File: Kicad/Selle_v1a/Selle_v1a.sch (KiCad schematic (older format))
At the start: 0 parts

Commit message: Update Schematic
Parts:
- added C1: 10u, symbol Device:CP1
- added C2: 100u, symbol Device:CP1
- added C3, C4: 100n, symbol Device:C
- added D1: D_Schottky_AKA, symbol Device:D_Schottky_AKA
- added IC1: R-785.0-0.5, RECOM_R-785.0-0.5, symbol R-785.0-0.5:R-785.0-0.5
- added IC2: MCP2562, Package_SO:SOIC-8_3.9x4.9mm_P1.27mm, symbol Interface_CAN_LIN:MCP2562-E-SN
- added K1: ALIM, symbol Connector_Generic:Conn_01x02
- added K2: BUS CAN, symbol Connector_Generic:Conn_01x02
- added R1: 120, symbol Device:R
- added UC1: BluePill STM32, symbol YAAJ_STM32:BluePill_1
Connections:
- new net: IC2.6 (CANL), K2.2 (Pin_2), R1.2
- new net: IC2.7 (CANH), K2.1 (Pin_1), R1.1
- new net: C1.1, D1.2 (K), IC1.1 (+VIN)
- new net: D1.1 (A), D1.3 (A), K1.1 (Pin_1)
- new net +5V: C2.1, C4.2, IC1.3 (+VOUT), IC2.3 (VDD), UC1.18 (5V)
- new net CANRX: IC2.4 (RXD), UC1.8 (PA11)
- new net CANTX: IC2.1 (TXD), UC1.9 (PA12)
- new net GND: C1.2, C2.2, C3.2, C4.1, IC1.2 (GND), IC2.2 (VSS), IC2.8 (STBY), K1.2 (Pin_2), UC1.19 (GND), UC1.39 (GND), UC1.40 (GND)
- new net SCL: UC1.14 (PB6)
- new net SDA: UC1.15 (PB7)
- new net VCC: C3.1, IC2.5 (Vio), UC1.20 (3V3)

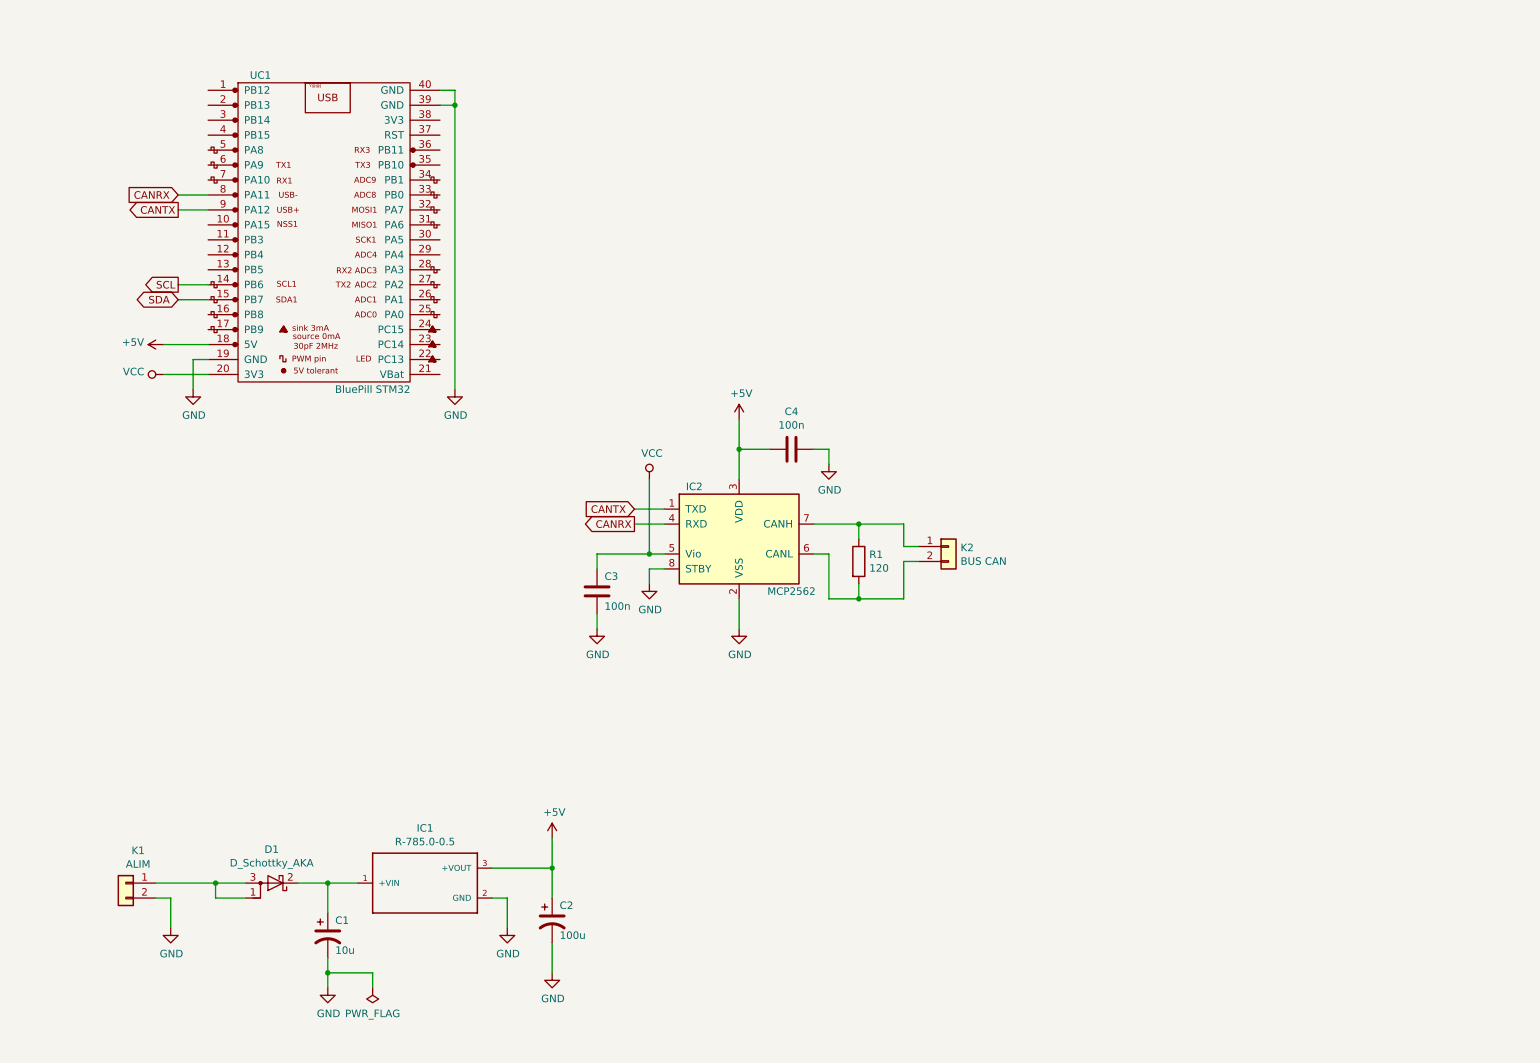
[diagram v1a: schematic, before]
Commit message: Update projet
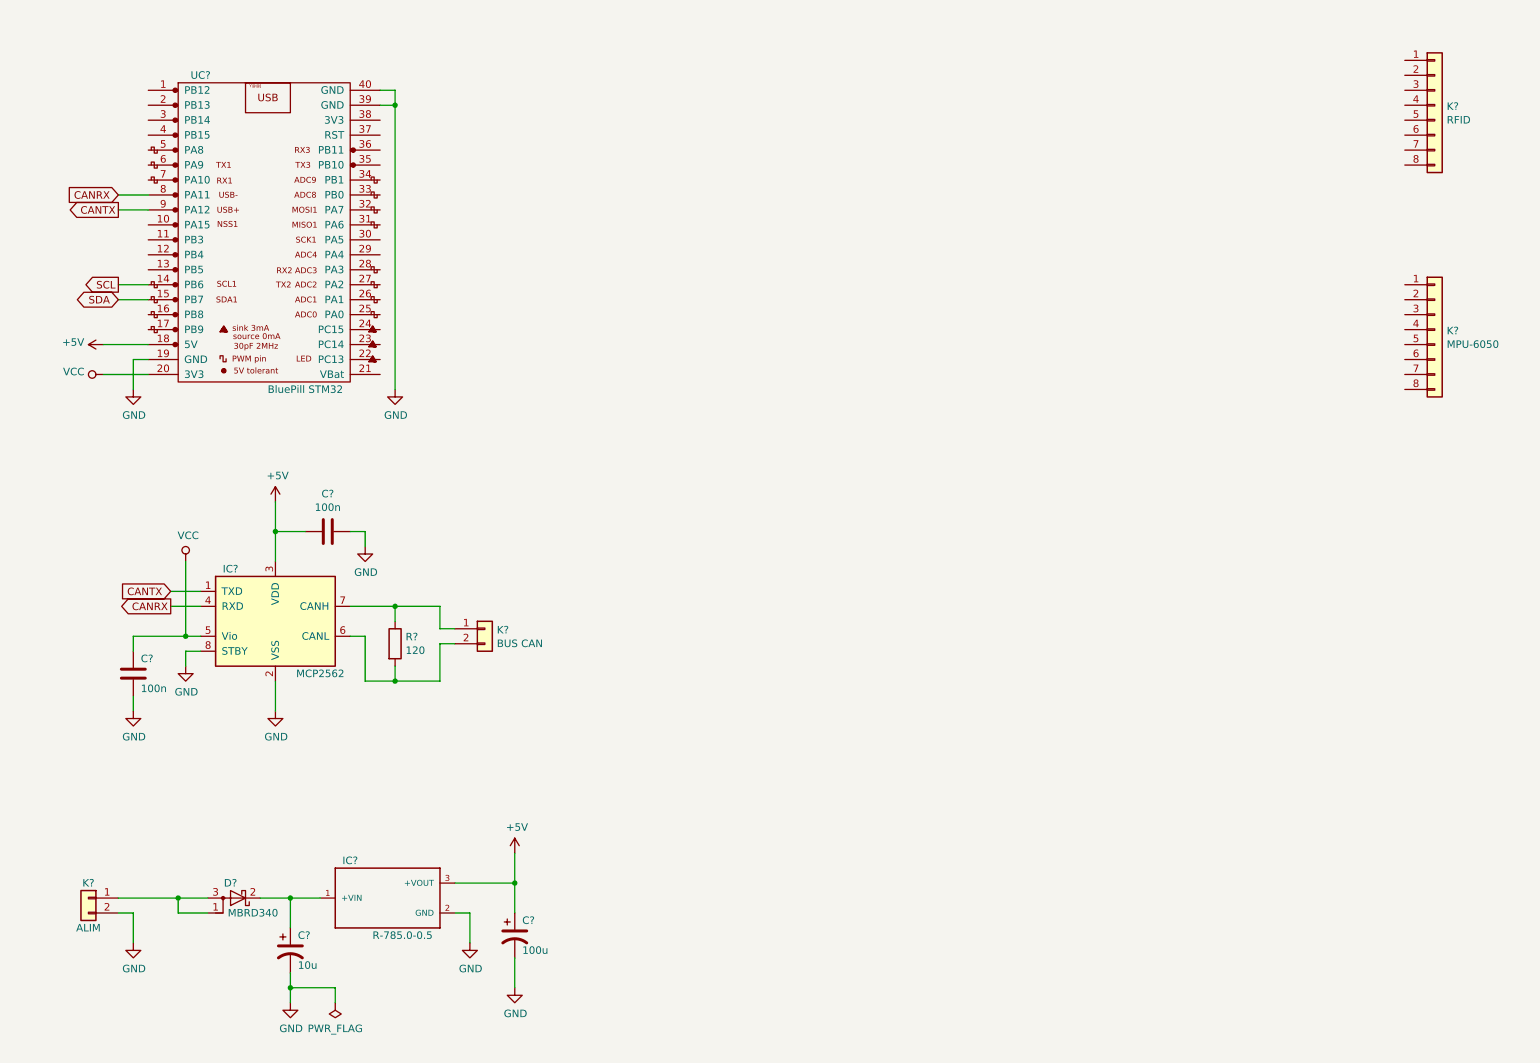
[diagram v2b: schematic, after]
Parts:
- added K?: RFID, symbol Connector_Generic:Conn_01x08
- added K?: MPU-6050, symbol Connector_Generic:Conn_01x08
- D?: renamed from D1; value D_Schottky_AKA -> MBRD340
- renumbered C4 to C?, C3 to C?, C1 to C?, C2 to C?, IC2 to IC?, IC1 to IC?, K1 to K?, K2 to K?, R1 to R?, UC1 to UC?
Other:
- moved on the sheet: C?, D?, IC?, K?, R?, UC?

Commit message: Update Schema
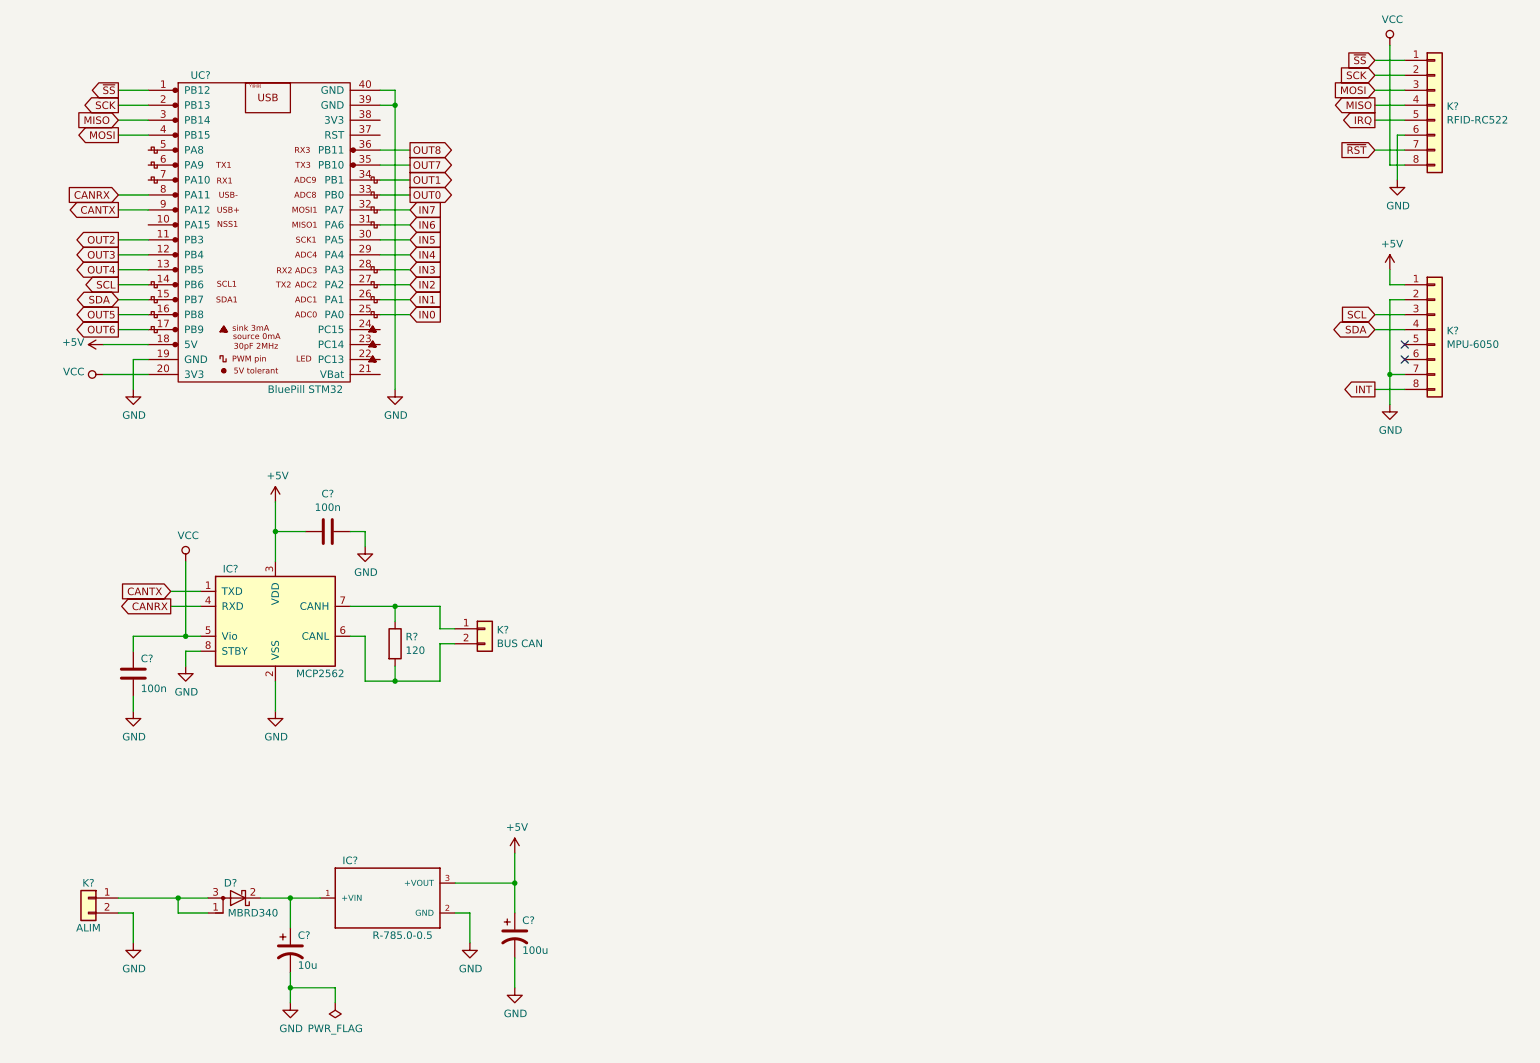
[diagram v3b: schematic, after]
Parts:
- K?: value RFID -> RFID-RC522
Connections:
- net +5V: now also K?.1 (Pin_1)
- net GND: now also K?.2 (Pin_2), K?.6 (Pin_6), K?.7 (Pin_7)
- net SCL: now also K?.3 (Pin_3)
- net SDA: now also K?.4 (Pin_4)
- net VCC: now also K?.8 (Pin_8)
- net ~SS: now reaches K?.1 (Pin_1)
- net ~SS: now also UC?.1 (PB12)
- net SCK: now reaches K?.2 (Pin_2)
- net SCK: now also UC?.2 (PB13)
- net MOSI: now reaches K?.3 (Pin_3)
- net MOSI: now also UC?.4 (PB15)
- net MISO: now reaches K?.4 (Pin_4)
- net MISO: now also UC?.3 (PB14)
- net IRQ: now reaches K?.5 (Pin_5)
- net ~RST: now reaches K?.7 (Pin_7)
- net INT: now reaches K?.8 (Pin_8)
- net OUT2: now reaches UC?.11 (PB3)
- net OUT3: now reaches UC?.12 (PB4)
- net OUT4: now reaches UC?.13 (PB5)
- net OUT5: now reaches UC?.16 (PB8)
- net OUT6: now reaches UC?.17 (PB9)
- net IN0: now reaches UC?.25 (PA0)
- net IN1: now reaches UC?.26 (PA1)
- net IN2: now reaches UC?.27 (PA2)
- net IN3: now reaches UC?.28 (PA3)
- net IN4: now reaches UC?.29 (PA4)
- net IN5: now reaches UC?.30 (PA5)
- net IN6: now reaches UC?.31 (PA6)
- net IN7: now reaches UC?.32 (PA7)
- net OUT0: now reaches UC?.33 (PB0)
- net OUT1: now reaches UC?.34 (PB1)
- net OUT7: now reaches UC?.35 (PB10)
- net OUT8: now reaches UC?.36 (PB11)
- no-connect marks 0 -> 2
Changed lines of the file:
@@
 P 10200 1300
 F 0 "K?" H 10280 1292 50  0000 L CNN
-F 1 "RFID" H 10280 1201 50  0000 L CNN
+F 1 "RFID-RC522" H 10280 1201 50  0000 L CNN
 F 2 "" H 10200 1300 50  0001 C CNN
 F 3 "~" H 10200 1300 50  0001 C CNN
@@
 	-1   0    0    1
 $EndComp
+Wire Wire Line
+	10000 1000 9800 1000
+Wire Wire Line
+	10000 1100 9800 1100
+Wire Wire Line
+	10000 1200 9800 1200
+Wire Wire Line
+	10000 1300 9800 1300
+$Comp
+L power:VCC #PWR?
+U 1 1 5E8C5F52
+P 9900 900
+F 0 "#PWR?" H 9900 750 50  0001 C CNN
+F 1 "VCC" H 9917 1073 50  0000 C CNN
+F 2 "" H 9900 900 50  0001 C CNN
+F 3 "" H 9900 900 50  0001 C CNN
+	1    9900 900
+	1    0    0    -1
+$EndComp
+$Comp
+L power:GND #PWR?
+U 1 1 5E8C663C
+P 9950 1800
+F 0 "#PWR?" H 9950 1550 50  0001 C CNN
+F 1 "GND" H 9955 1627 50  0000 C CNN
+F 2 "" H 9950 1800 50  0001 C CNN
+F 3 "" H 9950 1800 50  0001 C CNN
+	1    9950 1800
+	1    0    0    -1
+$EndComp
+Wire Wire Line
+	10000 1700 9900 1700
+Wire Wire Line
+	9900 1700 9900 900
+Wire Wire Line
+	10000 1500 9950 1500
+Wire Wire Line
+	9950 1500 9950 1800
+Wire Wire Line
+	10000 1600 9800 1600
+Text GLabel 9800 1000 0    50   Input ~ 0
+~SS
+Wire Wire Line
+	10000 1400 9800 1400
+Text GLabel 9800 1400 0    50   Output ~ 0
+IRQ
+Text GLabel 9800 1100 0    50   Input ~ 0
+SCK
+Text GLabel 9800 1200 0    50   Input ~ 0
+MOSI
+Text GLabel 9800 1300 0    50   Output ~ 0
+MISO
+Text GLabel 9800 1600 0    50   Input ~ 0
+~RST
+Wire Wire Line
+	1600 1500 1400 1500
+Wire Wire Line
+	1600 1400 1400 1400
+Wire Wire Line
+	1600 1300 1400 1300
+Wire Wire Line
+	1600 1200 1400 1200
+Text GLabel 1400 1200 0    50   Output ~ 0
+~SS
+Text GLabel 1400 1300 0    50   Output ~ 0
+SCK
+Text GLabel 1400 1400 0    50   Input ~ 0
+MISO
+Text GLabel 1400 1500 0    50   Output ~ 0
+MOSI
+$Comp
+L power:+5V #PWR?
+U 1 1 5E8DDE10
+P 9900 2400
+F 0 "#PWR?" H 9900 2250 50  0001 C CNN
+F 1 "+5V" H 9915 2573 50  0000 C CNN
+F 2 "" H 9900 2400 50  0001 C CNN
+F 3 "" H 9900 2400 50  0001 C CNN
+	1    9900 2400
+	1    0    0    -1
+$EndComp
+Wire Wire Line
+	10000 2500 9900 2500
+Wire Wire Line
+	9900 2500 9900 2400
+$Comp
+L power:GND #PWR?
+U 1 1 5E8DFFF4
+P 9900 3300
+F 0 "#PWR?" H 9900 3050 50  0001 C CNN
+F 1 "GND" H 9905 3127 50  0000 C CNN
+F 2 "" H 9900 3300 50  0001 C CNN
+F 3 "" H 9900 3300 50  0001 C CNN
+	1    9900 3300
+	1    0    0    -1
+$EndComp
+Wire Wire Line
+	10000 2700 9800 2700
+Wire Wire Line
+	10000 2800 9800 2800
+Wire Wire Line
+	10000 3200 9800 3200
+Text GLabel 9800 2700 0    50   Input ~ 0
+SCL
+Text GLabel 9800 2800 0    50   BiDi ~ 0
+SDA
+Text GLabel 9800 3200 0    50   Output ~ 0
+INT
+NoConn ~ 10000 2900
+NoConn ~ 10000 3000
+Wire Wire Line
+	10000 2600 9900 2600
+Wire Wire Line
+	9900 2600 9900 3100
+Wire Wire Line
+	10000 3100 9900 3100
+Connection ~ 9900 3100
+Wire Wire Line
+	9900 3100 9900 3300
+Wire Wire Line
+	3150 2700 3350 2700
+Wire Wire Line
+	3150 2600 3350 2600
+Wire Wire Line
+	3150 2500 3350 2500
+Wire Wire Line
+	3150 2400 3350 2400
+Wire Wire Line
+	3150 2300 3350 2300
+Wire Wire Line
+	3150 2200 3350 2200
+Wire Wire Line
+	3150 2100 3350 2100
+Wire Wire Line
+	3150 2000 3350 2000
+Text GLabel 3350 2700 2    50   Input ~ 0
+IN0
+Text GLabel 3350 2600 2    50   Input ~ 0
+IN1
+Text GLabel 3350 2500 2    50   Input ~ 0
+IN2
+Text GLabel 3350 2400 2    50   Input ~ 0
+IN3
+Text GLabel 3350 2300 2    50   Input ~ 0
+IN4
+Text GLabel 3350 2200 2    50   Input ~ 0
+IN5
+Text GLabel 3350 2100 2    50   Input ~ 0
+IN6
+Text GLabel 3350 2000 2    50   Input ~ 0
+IN7
+Wire Wire Line
+	3150 1900 3350 1900
+Wire Wire Line
+	3150 1800 3350 1800
+Wire Wire Line
+	1600 2200 1400 2200
+Wire Wire Line
+	1600 2300 1400 2300
+Wire Wire Line
+	1600 2400 1400 2400
+Wire Wire Line
+	1600 2700 1400 2700
+Wire Wire Line
+	1600 2800 1400 2800
+Wire Wire Line
+	3150 1700 3350 1700
+Wire Wire Line
+	3150 1600 3350 1600
+Text GLabel 3350 1900 2    50   Output ~ 0
+OUT0
+Text GLabel 3350 1800 2    50   Output ~ 0
+OUT1
+Text GLabel 1400 2200 0    50   Output ~ 0
+OUT2
+Text GLabel 1400 2300 0    50   Output ~ 0
+OUT3
+Text GLabel 1400 2400 0    50   Output ~ 0
+OUT4
+Text GLabel 1400 2700 0    50   Output ~ 0
+OUT5
+Text GLabel 1400 2800 0    50   Output ~ 0
+OUT6
+Text GLabel 3350 1700 2    50   Output ~ 0
+OUT7
+Text GLabel 3350 1600 2    50   Output ~ 0
+OUT8
 $EndSCHEMATC

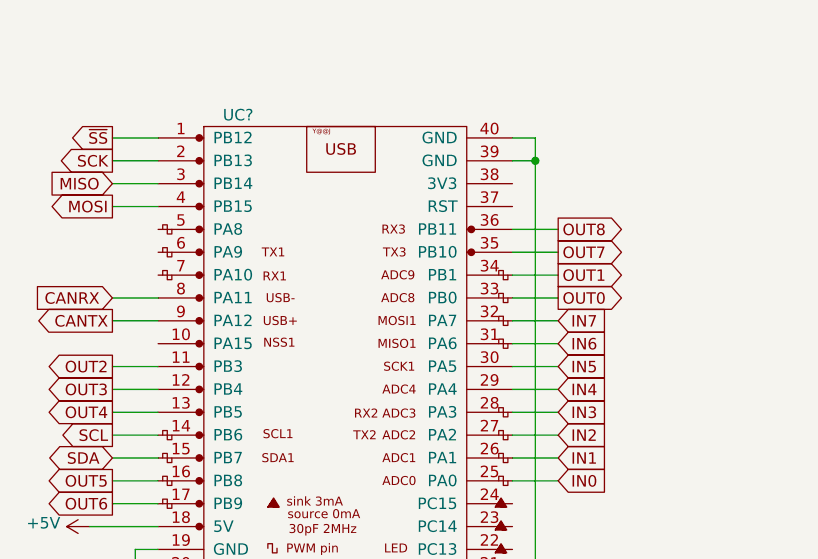
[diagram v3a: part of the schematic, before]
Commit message: Update schema
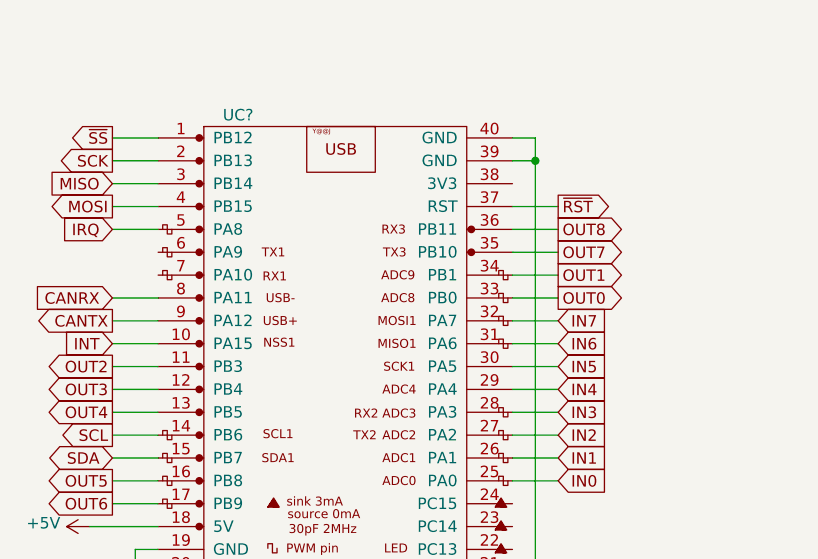
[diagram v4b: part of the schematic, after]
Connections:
- net INT: now also UC?.10 (PA15)
- net IRQ: now also UC?.5 (PA8)
- net ~RST: now also UC?.37 (RST)
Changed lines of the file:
@@
 Text GLabel 3350 1600 2    50   Output ~ 0
 OUT8
+Wire Wire Line
+	1600 1600 1400 1600
+Text GLabel 1400 1600 0    50   Input ~ 0
+IRQ
+Wire Wire Line
+	3150 1500 3350 1500
+Text GLabel 3350 1500 2    50   Output ~ 0
+~RST
+Wire Wire Line
+	1600 2100 1400 2100
+Text GLabel 1400 2100 0    50   Input ~ 0
+INT
 $EndSCHEMATC
